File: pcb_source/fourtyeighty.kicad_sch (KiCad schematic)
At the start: 148 parts, among them J1 USB_C_Receptacle_USB2.0, SW1 RotaryEncoder_Switch, U1 XC6206PxxxMR, U2 SRV05-4, U3 W25Q128JVS, U4 RP2040TR7, Y1 Crystal_GND24_Small

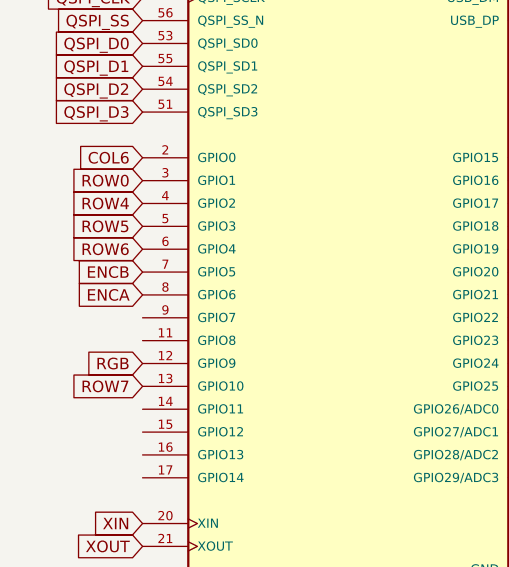
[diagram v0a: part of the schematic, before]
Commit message: Just a few more connections
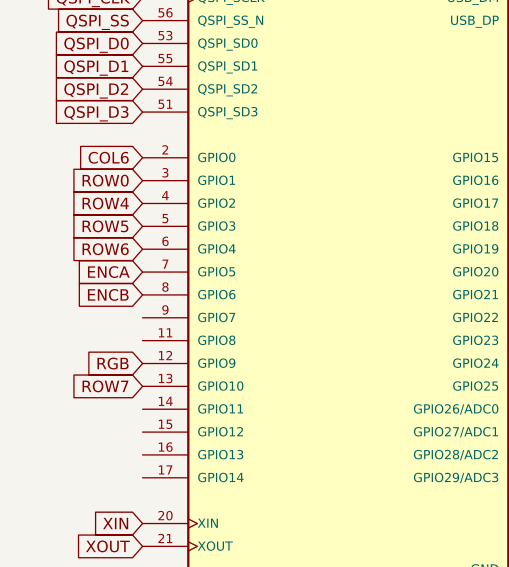
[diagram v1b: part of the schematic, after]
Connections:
- net ENCA: now also U4.7 (GPIO5); no longer U4.8 (GPIO6)
- net ENCB: now also U4.8 (GPIO6); no longer U4.7 (GPIO5)
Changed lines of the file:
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@@
     )
   )
-  (global_label "ENCB" (shape input) (at 29.21 151.13 180) (fields_autoplaced)
-    (effects (font (size 1.27 1.27)) (justify right))
-    (property "Intersheetrefs" "${INTERSHEET_REFS}" (at 21.2847 151.13 0)
+  (global_label "ENCB" (shape input) (at 29.21 153.67 180) (fields_autoplaced)
+    (effects (font (size 1.27 1.27)) (justify right))
+    (property "Intersheetrefs" "${INTERSHEET_REFS}" (at 21.2847 153.67 0)
       (effects (font (size 1.27 1.27)) (justify right) hide)
     )
@@
     )
   )
-  (global_label "ENCA" (shape input) (at 29.21 153.67 180) (fields_autoplaced)
-    (effects (font (size 1.27 1.27)) (justify right))
-    (property "Intersheetrefs" "${INTERSHEET_REFS}" (at 21.4661 153.67 0)
-      (effects (font (size 1.27 1.27)) (justify right) hide)
-    )
+  (global_label "ENCA" (shape input) (at 29.21 151.13 180) (fields_autoplaced)
+    (effects (font (size 1.27 1.27)) (justify right))
+    (property "Intersheetrefs" "${INTERSHEET_REFS}" (at 21.4661 151.13 0)
+      (effects (font (size 1.27 1.27)) (justify right) hide)
+    )
